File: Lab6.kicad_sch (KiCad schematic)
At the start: 32 parts, among them J1 JTAG, J2 Battery, SW1 Reset, SW2 Input, U1 TM4C123GH6PMIR, U2 Adafruit ST7735R, U3 LP2950-33LPRE3, Y1 ABM3-16.000MHZ-B2-T

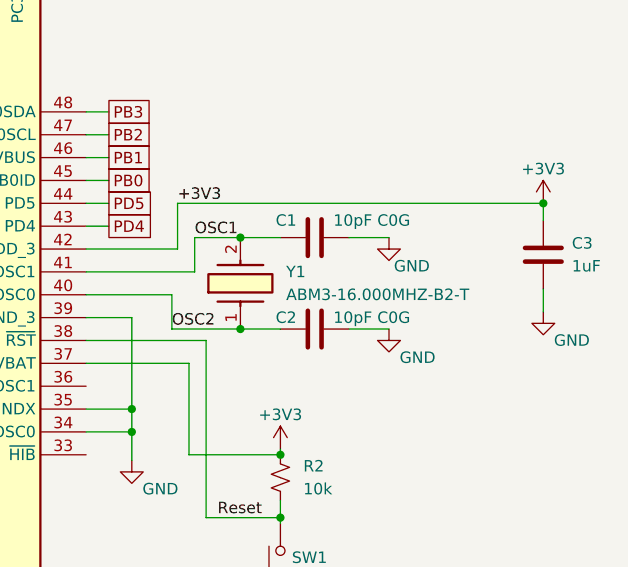
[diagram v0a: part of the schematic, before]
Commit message: Valvano Dump
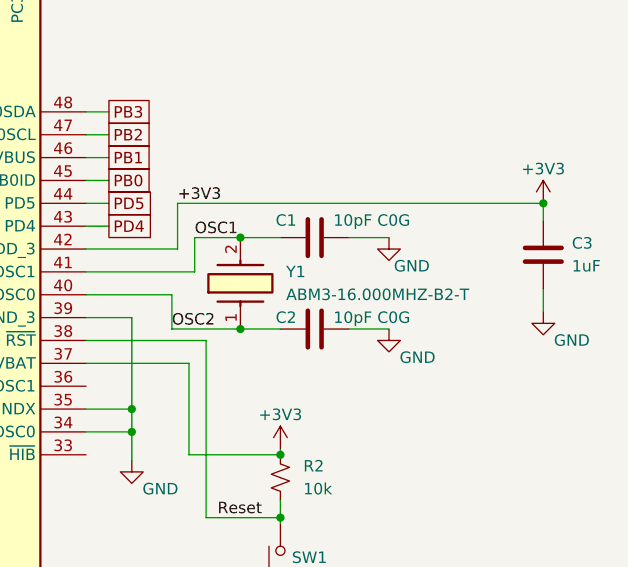
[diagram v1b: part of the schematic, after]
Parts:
- U1: symbol TM4C123GH6PMIR:TM4C123GH6PMIR -> ECE445L:TM4C123GH6PMIR
- U3: symbol LP2950-33LPRE3:LP2950-33LPRE3 -> ECE445L:LP2950-33LPRE3
- Y1: symbol ABM3-16_000MHZ-B2-T:ABM3-16.000MHZ-B2-T -> ECE445L:ABM3-16.000MHZ-B2-T
